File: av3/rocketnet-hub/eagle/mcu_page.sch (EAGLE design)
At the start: 331 parts, among them J1 ROCKETBUS, J2 ROCKETBUS, J3 ROCKETBUS, J4 ROCKETBUS, J5 ROCKETBUS, J6 ROCKETBUS, J7 ROCKETBUS, J8 ROCKETBUS, X1 87758-0416, X2 87758-0416, X3 87758-0416, X4 87758-0416, X5 87758-0416, X6 87758-0416, X7 87758-0416, X8 87758-0416

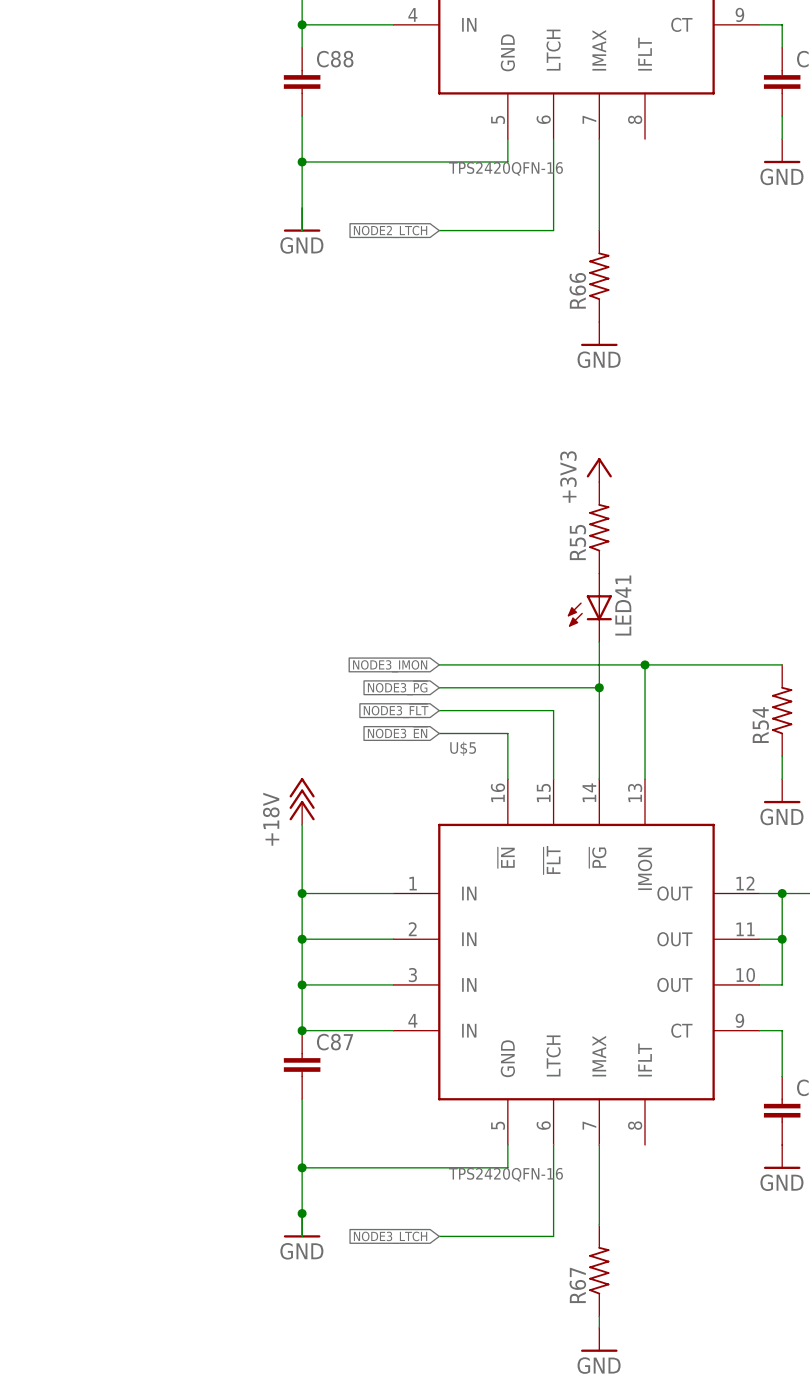
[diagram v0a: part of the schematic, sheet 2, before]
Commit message: Rearranged the layout of switch circuit - work in progress
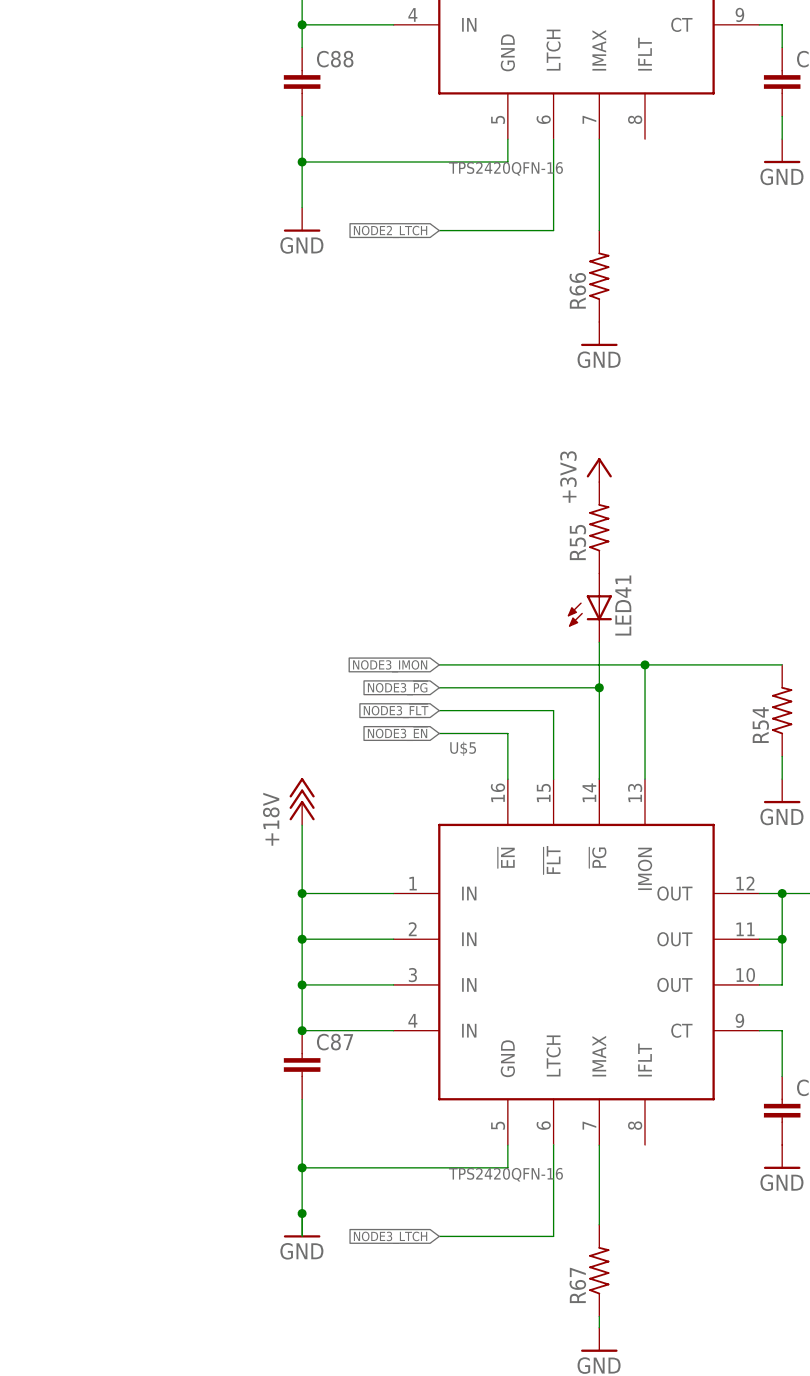
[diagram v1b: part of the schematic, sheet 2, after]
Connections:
- net N$141 renamed RATSNET
- removed net N$123: C88.2, U$4.GND@5
- removed net N$124: C87.2, U$5.GND@5
- net GND: now also C87.2, C88.2, U$4.GND@5, U$5.GND@5
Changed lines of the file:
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@@
 <wire x1="27.94" y1="111.76" x2="27.94" y2="114.3" width="0.1524" layer="91"/>
 <pinref part="GND45" gate="1" pin="GND"/>
-<wire x1="27.94" y1="114.3" x2="27.94" y2="119.38" width="0.1524" layer="91"/>
 <junction x="27.94" y="114.3"/>
+<wire x1="50.8" y1="121.92" x2="50.8" y2="119.38" width="0.1524" layer="91"/>
+<pinref part="U$5" gate="G$1" pin="GND@5"/>
+<wire x1="50.8" y1="119.38" x2="27.94" y2="119.38" width="0.1524" layer="91"/>
+<wire x1="27.94" y1="119.38" x2="27.94" y2="114.3" width="0.1524" layer="91"/>
+<pinref part="C87" gate="G$1" pin="2"/>
+<wire x1="27.94" y1="119.38" x2="27.94" y2="127" width="0.1524" layer="91"/>
+<junction x="27.94" y="119.38"/>
 </segment>
 <segment>
@@
 <pinref part="R72" gate="G$1" pin="1"/>
 <pinref part="GND62" gate="1" pin="GND"/>
+</segment>
+<segment>
+<wire x1="50.8" y1="233.68" x2="50.8" y2="231.14" width="0.1524" layer="91"/>
+<pinref part="C88" gate="G$1" pin="2"/>
+<wire x1="27.94" y1="236.22" x2="27.94" y2="231.14" width="0.1524" layer="91"/>
+<wire x1="27.94" y1="231.14" x2="50.8" y2="231.14" width="0.1524" layer="91"/>
+<pinref part="U$4" gate="G$1" pin="GND@5"/>
+<pinref part="GND44" gate="1" pin="GND"/>
+<wire x1="27.94" y1="226.06" x2="27.94" y2="231.14" width="0.1524" layer="91"/>
+<junction x="27.94" y="231.14"/>
 </segment>
 </net>
@@
 </segment>
 </net>
-<net name="N$123" class="0">
-<segment>
-<wire x1="50.8" y1="233.68" x2="50.8" y2="231.14" width="0.1524" layer="91"/>
-<pinref part="C88" gate="G$1" pin="2"/>
-<wire x1="27.94" y1="236.22" x2="27.94" y2="231.14" width="0.1524" layer="91"/>
-<wire x1="27.94" y1="231.14" x2="50.8" y2="231.14" width="0.1524" layer="91"/>
-<pinref part="U$4" gate="G$1" pin="GND@5"/>
-<wire x1="27.94" y1="223.52" x2="27.94" y2="231.14" width="0.1524" layer="91"/>
-<junction x="27.94" y="231.14"/>
-</segment>
-</net>
-<net name="N$124" class="0">
-<segment>
-<wire x1="50.8" y1="121.92" x2="50.8" y2="119.38" width="0.1524" layer="91"/>
-<pinref part="C87" gate="G$1" pin="2"/>
-<wire x1="27.94" y1="127" x2="27.94" y2="119.38" width="0.1524" layer="91"/>
-<wire x1="27.94" y1="119.38" x2="50.8" y2="119.38" width="0.1524" layer="91"/>
-<pinref part="U$5" gate="G$1" pin="GND@5"/>
-<junction x="27.94" y="119.38"/>
-</segment>
-</net>
 <net name="N$126" class="0">
 <segment>
@@
 </segment>
 </net>
-<net name="N$141" class="0">
+<net name="RATSNET" class="0">
 <segment>
 <pinref part="C97" gate="G$1" pin="1"/>

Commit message: added vias to center pad to package
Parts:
- added U$26, U$27: MAX4734ETC+, max4734:MAX4734ETC+
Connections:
- new net N$30: U$26.GND
- new net N$31: U$26.COM
- net NODE1_IMON: now also U$26.N0
- net NODE2_IMON: now also U$26.N2
- net NODE3_IMON: now also U$26.N3
- net NODE4_IMON: now also U$26.N4
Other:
- moved on the sheet: U$10, U$3, U$4, U$5, U$6, U$7, U$8, U$9
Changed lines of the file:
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@@
 <part name="+3V17" library="supply1" deviceset="+3V3" device=""/>
 <part name="+3V18" library="supply1" deviceset="+3V3" device=""/>
+<part name="U$26" library="max4734" deviceset="MAX4734ETC+" device=""/>
+<part name="U$27" library="max4734" deviceset="MAX4734ETC+" device=""/>
 </parts>
 <sheets>
@@
 <instance part="P+8" gate="1" x="30.48" y="-309.88"/>
 <instance part="P+9" gate="1" x="30.48" y="-426.72"/>
+<instance part="U$26" gate="G$1" x="-30.48" y="195.58"/>
+<instance part="U$27" gate="G$1" x="-10.16" y="-276.86"/>
 </instances>
 <busses>
@@
 <wire x1="66.04" y1="406.4" x2="66.04" y2="419.1" width="0.1524" layer="91"/>
 <wire x1="66.04" y1="419.1" x2="81.28" y2="419.1" width="0.1524" layer="91"/>
-<wire x1="66.04" y1="419.1" x2="43.18" y2="419.1" width="0.1524" layer="91"/>
 <junction x="66.04" y="419.1"/>
 <pinref part="R49" gate="G$1" pin="2"/>
 <label x="43.18" y="419.1" size="1.016" layer="95" rot="R180" xref="yes"/>
+<pinref part="U$26" gate="G$1" pin="N0"/>
+<wire x1="-43.18" y1="198.12" x2="-45.72" y2="198.12" width="0.1524" layer="91"/>
+<wire x1="-45.72" y1="198.12" x2="-45.72" y2="419.1" width="0.1524" layer="91"/>
+<wire x1="-45.72" y1="419.1" x2="66.04" y2="419.1" width="0.1524" layer="91"/>
 </segment>
 </net>
@@
 <net name="NODE2_IMON" class="0">
 <segment>
-<wire x1="43.18" y1="287.02" x2="66.04" y2="287.02" width="0.1524" layer="91"/>
 <pinref part="U$4" gate="G$1" pin="IMON"/>
 <wire x1="66.04" y1="287.02" x2="66.04" y2="274.32" width="0.1524" layer="91"/>
@@
 <junction x="66.04" y="287.02"/>
 <label x="43.18" y="287.02" size="1.016" layer="95" rot="R180" xref="yes"/>
+<pinref part="U$26" gate="G$1" pin="N2"/>
+<wire x1="-17.78" y1="198.12" x2="-12.7" y2="198.12" width="0.1524" layer="91"/>
+<wire x1="-12.7" y1="198.12" x2="-12.7" y2="287.02" width="0.1524" layer="91"/>
+<wire x1="-12.7" y1="287.02" x2="66.04" y2="287.02" width="0.1524" layer="91"/>
 </segment>
 </net>
@@
 <pinref part="U$5" gate="G$1" pin="IMON"/>
 <wire x1="66.04" y1="162.56" x2="66.04" y2="175.26" width="0.1524" layer="91"/>
-<wire x1="66.04" y1="175.26" x2="43.18" y2="175.26" width="0.1524" layer="91"/>
 <pinref part="R54" gate="G$1" pin="2"/>
 <wire x1="66.04" y1="175.26" x2="81.28" y2="175.26" width="0.1524" layer="91"/>
 <junction x="66.04" y="175.26"/>
 <label x="43.18" y="175.26" size="1.016" layer="95" rot="R180" xref="yes"/>
+<pinref part="U$26" gate="G$1" pin="N3"/>
+<wire x1="-43.18" y1="193.04" x2="-45.72" y2="193.04" width="0.1524" layer="91"/>
+<wire x1="-45.72" y1="193.04" x2="-45.72" y2="175.26" width="0.1524" layer="91"/>
+<wire x1="-45.72" y1="175.26" x2="66.04" y2="175.26" width="0.1524" layer="91"/>
 </segment>
 </net>
@@
 <pinref part="R58" gate="G$1" pin="2"/>
 <wire x1="81.28" y1="53.34" x2="66.04" y2="53.34" width="0.1524" layer="91"/>
-<wire x1="66.04" y1="53.34" x2="43.18" y2="53.34" width="0.1524" layer="91"/>
 <label x="43.18" y="53.34" size="1.016" layer="95" rot="R180" xref="yes"/>
 <junction x="66.04" y="53.34"/>
+<pinref part="U$26" gate="G$1" pin="N4"/>
+<wire x1="-17.78" y1="193.04" x2="-12.7" y2="193.04" width="0.1524" layer="91"/>
+<wire x1="-12.7" y1="193.04" x2="-12.7" y2="53.34" width="0.1524" layer="91"/>
+<wire x1="-12.7" y1="53.34" x2="66.04" y2="53.34" width="0.1524" layer="91"/>
 </segment>
 </net>
@@
 </segment>
 </net>
+<net name="N$30" class="0">
+<segment>
+<pinref part="U$26" gate="G$1" pin="GND"/>
+<wire x1="-43.18" y1="195.58" x2="-50.8" y2="195.58" width="0.1524" layer="91"/>
+<wire x1="-50.8" y1="195.58" x2="-50.8" y2="185.42" width="0.1524" layer="91"/>
+</segment>
+</net>
+<net name="N$31" class="0">
+<segment>
+<pinref part="U$26" gate="G$1" pin="COM"/>
+<wire x1="-17.78" y1="195.58" x2="-5.08" y2="195.58" width="0.1524" layer="91"/>
+</segment>
+</net>
